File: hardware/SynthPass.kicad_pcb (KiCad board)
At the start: 4 copper layers, 31.5 x 18 mm, 19 parts, among them P1 USB_C_Plug_USB2.0, SW1 SW_Push, U2 CH572D, Y2 32MHz

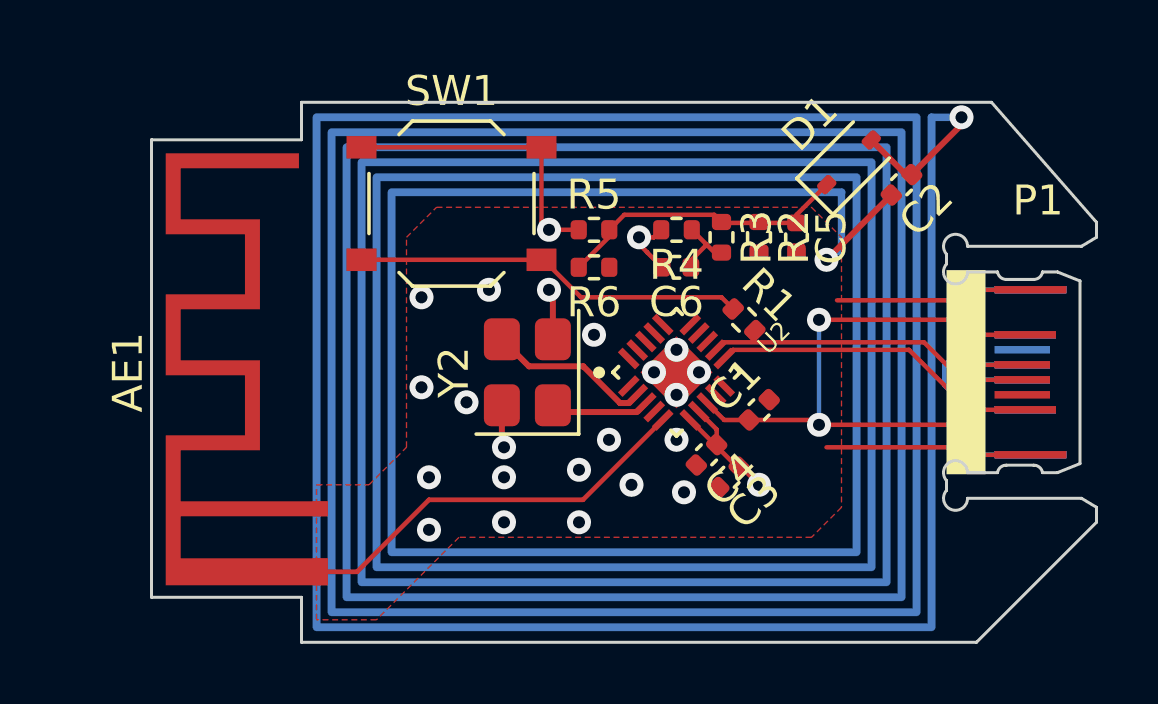
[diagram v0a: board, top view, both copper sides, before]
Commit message: Finalize hardware design, pending pinout confirmation
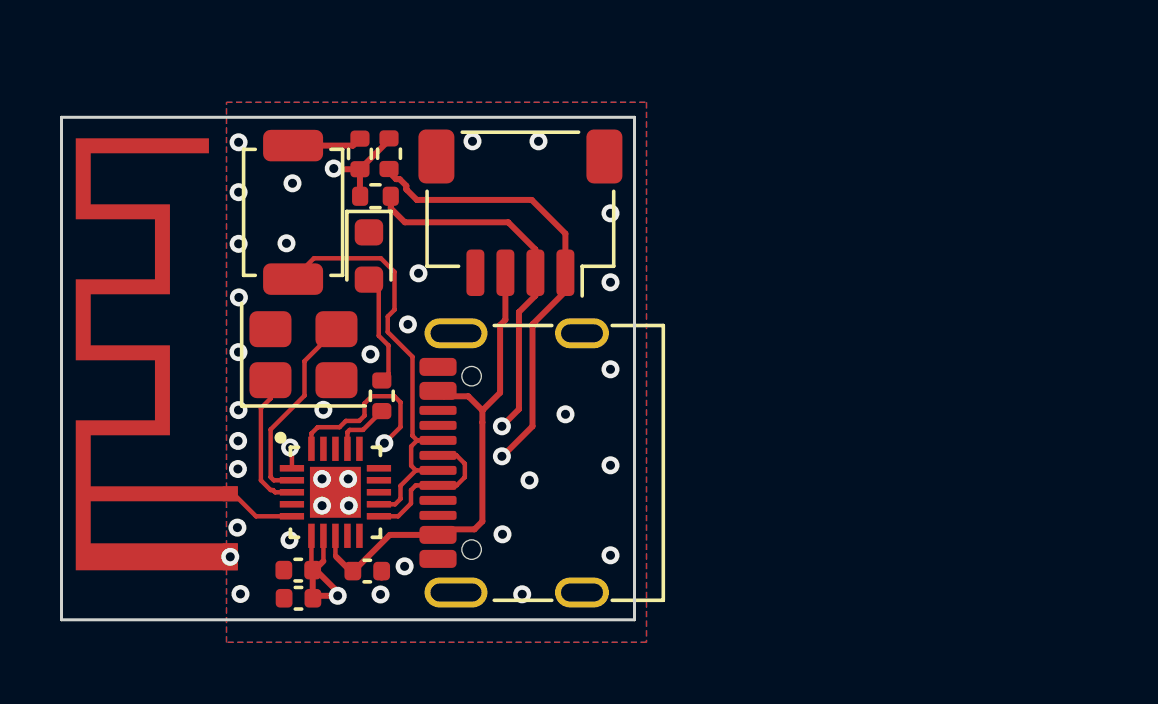
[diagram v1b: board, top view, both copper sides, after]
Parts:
- removed AE2: NFC, NFC_Antenna:Antenna_21x17_6T
- removed C2: 47p, Capacitor_SMD:C_0402_1005Metric
- removed C5: 220p, Capacitor_SMD:C_0402_1005Metric
- removed C6: 10n, Capacitor_SMD:C_0402_1005Metric
- removed R5: 100k, Resistor_SMD:R_0402_1005Metric
- removed R6: 1k, Resistor_SMD:R_0402_1005Metric
- added G***: LOGO, graphics:synthpass, B.Cu at (159.2, 57.9)
- added G***: LOGO, graphics:pretzel, B.Cu at (159.0, 64.3)
- added G***: LOGO, graphics:qr, B.Cu at (153.5, 61.8)
- added J1: SM04B-SRSS-TB, Connector_JST:JST_SH_SM04B-SRSS-TB_1x04-1MP_P1.00mm_Horizontal, F.Cu at (164.8, 52.7)
- D1: value 1N4148WS -> LED_Small; footprint Diode_SMD:D_SOD-323 -> LED_SMD:LED_0603_1608Metric
- P1: footprint PCM_PCB_USBC:PCBTypeC_14P -> Connector_USB:USB_C_Receptacle_G-Switch_GT-USB-7010ASV
- R1: value 1.5k -> 5.1k
- R2: value 1k -> 5.1k
- R3, R4: value 10k -> 5.1k
- SW1: footprint Button_Switch_SMD:SW_Push_1P1T_XKB_TS-1187A -> Button_Switch_SMD:SW_SPST_TS-1088-xR020
- moved D1 16.3 mm to (159.7, 54.1), turned to -90 degrees
- moved C3 14.9 mm to (157.4, 65.5), turned to 180 degrees
- moved C4 14.1 mm to (157.4, 64.6), turned to 180 degrees
- moved C1 14.1 mm to (159.7, 64.6), turned to 0 degrees
- moved R1 13.9 mm to (159.4, 50.7), turned to -90 degrees
- moved R2 13.6 mm to (160.2, 58.8), turned to 90 degrees
- moved U2 13.6 mm to (159.4, 64.1), turned to 0 degrees
- moved P1 13.6 mm to (165.8, 61.0), turned to 90 degrees
- moved R3 11.4 mm to (160.4, 50.7), turned to 90 degrees
- moved R4 10.1 mm to (160.0, 52.1)
- moved Y2 7.49 mm to (157.6, 57.4), turned to 0 degrees
- moved SW1 5.29 mm to (157.2, 52.7), turned to 90 degrees
- moved AE1 3.04 mm to (155.1, 62.0)
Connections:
- AE1 pad 1: GND -> Net-(AE1-FEED)
- AE1 pad 2: Net-(AE1-PCB_Trace) -> GND
- D1 pad 1: Net-(D1-K) -> GND
- R1 pad 2: UDP -> +3V3
- R2 pad 1: Net-(D1-K) -> Net-(U2-PA10/R6/T7)
- R2 pad 2: GND -> Net-(D1-A)
- R3 pad 1: Net-(D1-K) -> SCL
- R3 pad 2: ENV -> +3V3
- R4 pad 1: ENV -> SDA
- R4 pad 2: GND -> +3V3
- SW1 pad 1: +3V3 -> UDP
- U2 pad 1: unconnected-(U2-PA3/T/R1/SCL2/SCK_/PWM3/CP0-Pad1) -> SCL
- U2 pad 16: unconnected-(U2-PA7/MOSI/T4/PWM1/TMR/RST_/CP1-Pad16) -> LED
- U2 pad 17: unconnected-(U2-PA10/R6/T7-Pad17) -> Net-(U2-PA10/R6/T7)
- U2 pad 20: unconnected-(U2-PA2/R/T1/SDA2/SCS_/PWM2/TMR1/CN-Pad20) -> SDA
- U2 pad 5: Net-(AE1-PCB_Trace) -> Net-(AE1-FEED)
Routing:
- net GND: track 24.1 -> 0.22 mm, vias 25 -> 35
- net SCL: track 0.00 -> 23.7 mm, vias 0 -> 2
- net SDA: track 0.00 -> 22.3 mm, vias 0 -> 2
- net Net-(AE1-PCB_Trace): track 14.1 -> 0.00 mm
- net Net-(R1-Pad1): track 13.1 -> 2.40 mm
- net Net-(D1-K): track 9.93 -> 0.00 mm
- net UDM: track 14.1 -> 5.00 mm, vias 2 -> 0
- net +3V3: track 14.3 -> 8.77 mm
- net UDP: track 11.5 -> 14.5 mm, vias 1 -> 0
- net VBUS: track 19.9 -> 16.9 mm, vias 2 -> 0
- net Net-(AE1-FEED): track 0.00 -> 2.37 mm
- net ENV: track 2.28 -> 0.00 mm
- net Net-(U2-PA10/R6/T7): track 0.00 -> 1.99 mm
- net Net-(U2-XI): track 3.31 -> 4.68 mm
- net Net-(D1-A): track 4.92 -> 3.73 mm, vias 1 -> 0
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- added copper zone on B.Cu, net GND
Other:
- board size 31.5 x 18 mm -> 19.1 x 16.8 mm
- board text added: "EL's"
- board text added: "LAB"
- board text added: "PASS"
- board text added: "PRET"
- board text added: "R1"
- board text added: "SYNTH"
- board text added: "Z"
